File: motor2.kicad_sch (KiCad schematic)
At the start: 58 parts, among them IC5 DRV8300DPWR, IC6 DRV8300DPWR, J10 Conn_01x01, J11 Conn_01x01, J12 Conn_01x01, J7 Conn_01x01, J8 Conn_01x01, J9 Conn_01x01, Q13 Q_NMOS, Q14 Q_NMOS, Q15 Q_NMOS, Q16 Q_NMOS, Q17 Q_NMOS, Q18 Q_NMOS, Q19 Q_NMOS, Q20 Q_NMOS, Q21 Q_NMOS, Q22 Q_NMOS, Q23 Q_NMOS, Q24 Q_NMOS

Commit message: affected footprints
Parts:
- C21, C23, C24, C25, C26, C27, C28, C29: footprint (none) -> Capacitor_SMD:C_0402_1005Metric
- J10, J11, J12, J7, J8, J9: footprint (none) -> TestPoint:TestPoint_Pad_2.0x2.0mm; now left out of the parts list
- Q13, Q14, Q15, Q16, Q17, Q18, Q19, Q20, Q21, Q22, Q23, Q24: footprint (none) -> ESCs:TRANS_NTMFS5C628NLT1G
- R42, R43, R44, R45, R46, R47, R48, R49, R50, R51, R52, R53, R54, R55, R56, R57, R58, R59, R60, R61, R62, R63, R64, R65, R66, R67, R68, R69, R70, R71: footprint (none) -> Resistor_SMD:R_0402_1005Metric
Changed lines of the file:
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@@
 			)
 		)
-		(property "Footprint" ""
+		(property "Footprint" "Resistor_SMD:R_0402_1005Metric"
 			(at 181.61 42.418 90)
 			(effects
@@
 			)
 		)
-		(property "Footprint" ""
+		(property "Footprint" "ESCs:TRANS_NTMFS5C628NLT1G"
 			(at 129.54 130.81 0)
 			(effects
@@
 			)
 		)
-		(property "Footprint" ""
+		(property "Footprint" "ESCs:TRANS_NTMFS5C628NLT1G"
 			(at 129.54 115.57 0)
 			(effects
@@
 			)
 		)
-		(property "Footprint" ""
+		(property "Footprint" "Resistor_SMD:R_0402_1005Metric"
 			(at 66.548 71.12 90)
 			(effects
@@
 			)
 		)
-		(property "Footprint" ""
+		(property "Footprint" "Resistor_SMD:R_0402_1005Metric"
 			(at 112.268 81.28 90)
 			(effects
@@
 			)
 		)
-		(property "Footprint" ""
+		(property "Footprint" "Resistor_SMD:R_0402_1005Metric"
 			(at 157.48 135.128 90)
 			(effects
@@
 			)
 		)
-		(property "Footprint" ""
+		(property "Footprint" "Resistor_SMD:R_0402_1005Metric"
 			(at 199.39 119.888 90)
 			(effects
@@
 			)
 		)
-		(property "Footprint" ""
+		(property "Footprint" "ESCs:TRANS_NTMFS5C628NLT1G"
 			(at 214.63 115.57 0)
 			(effects
@@
 			)
 		)
-		(property "Footprint" ""
+		(property "Footprint" "Resistor_SMD:R_0402_1005Metric"
 			(at 57.658 158.75 90)
 			(effects
@@
 			)
 		)
-		(property "Footprint" ""
+		(property "Footprint" "Resistor_SMD:R_0402_1005Metric"
 			(at 38.1 162.052 90)
 			(effects
@@
 			)
 		)
-		(property "Footprint" ""
+		(property "Footprint" "ESCs:TRANS_NTMFS5C628NLT1G"
 			(at 214.63 130.81 0)
 			(effects
@@
 		(unit 1)
 		(exclude_from_sim no)
-		(in_bom yes)
+		(in_bom no)
 		(on_board yes)
 		(dnp no)
@@
 			)
 		)
-		(property "Footprint" ""
+		(property "Footprint" "TestPoint:TestPoint_Pad_2.0x2.0mm"
 			(at 176.53 125.73 0)
 			(effects
@@
 			)
 		)
-		(property "Footprint" ""
+		(property "Footprint" "Resistor_SMD:R_0402_1005Metric"
 			(at 34.798 158.75 90)
 			(effects
@@
 			)
 		)
-		(property "Footprint" ""
+		(property "Footprint" "Capacitor_SMD:C_0402_1005Metric"
 			(at 85.09 105.7148 0)
 			(effects
@@
 			)
 		)
-		(property "Footprint" ""
+		(property "Footprint" "Capacitor_SMD:C_0402_1005Metric"
 			(at 85.09 113.3348 0)
 			(effects
@@
 			)
 		)
-		(property "Footprint" ""
+		(property "Footprint" "ESCs:TRANS_NTMFS5C628NLT1G"
 			(at 238.76 38.1 0)
 			(effects
@@
 			)
 		)
-		(property "Footprint" ""
+		(property "Footprint" "Resistor_SMD:R_0402_1005Metric"
 			(at 115.57 74.422 90)
 			(effects
@@
 		(unit 1)
 		(exclude_from_sim no)
-		(in_bom yes)
+		(in_bom no)
 		(on_board yes)
 		(dnp no)
@@
 			)
 		)
-		(property "Footprint" ""
+		(property "Footprint" "TestPoint:TestPoint_Pad_2.0x2.0mm"
 			(at 200.66 48.26 0)
 			(effects
@@
 			)
 		)
-		(property "Footprint" ""
+		(property "Footprint" "Resistor_SMD:R_0402_1005Metric"
 			(at 60.96 162.052 90)
 			(effects
@@
 		(unit 1)
 		(exclude_from_sim no)
-		(in_bom yes)
+		(in_bom no)
 		(on_board yes)
 		(dnp no)
@@
 			)
 		)
-		(property "Footprint" ""
+		(property "Footprint" "TestPoint:TestPoint_Pad_2.0x2.0mm"
 			(at 133.35 125.73 0)
 			(effects
@@
 		(unit 1)
 		(exclude_from_sim no)
-		(in_bom yes)
+		(in_bom no)
 		(on_board yes)
 		(dnp no)
@@
 			)
 		)
-		(property "Footprint" ""
+		(property "Footprint" "TestPoint:TestPoint_Pad_2.0x2.0mm"
 			(at 218.44 125.73 0)
 			(effects
@@
 			)
 		)
-		(property "Footprint" ""
+		(property "Footprint" "Resistor_SMD:R_0402_1005Metric"
 			(at 157.48 119.888 90)
 			(effects
@@
 			)
 		)
-		(property "Footprint" ""
+		(property "Footprint" "ESCs:TRANS_NTMFS5C628NLT1G"
 			(at 153.67 38.1 0)
 			(effects
@@
 			)
 		)
-		(property "Footprint" ""
+		(property "Footprint" "Resistor_SMD:R_0402_1005Metric"
 			(at 57.658 168.91 90)
 			(effects
@@
 			)
 		)
-		(property "Footprint" ""
+		(property "Footprint" "Resistor_SMD:R_0402_1005Metric"
 			(at 138.43 42.418 90)
 			(effects
@@
 			)
 		)
-		(property "Footprint" ""
+		(property "Footprint" "Resistor_SMD:R_0402_1005Metric"
 			(at 80.518 168.91 90)
 			(effects
@@
 			)
 		)
-		(property "Footprint" ""
+		(property "Footprint" "Resistor_SMD:R_0402_1005Metric"
 			(at 114.3 135.128 90)
 			(effects
@@
 			)
 		)
-		(property "Footprint" ""
+		(property "Footprint" "Resistor_SMD:R_0402_1005Metric"
 			(at 89.408 81.28 90)
 			(effects
@@
 			)
 		)
-		(property "Footprint" ""
+		(property "Footprint" "ESCs:TRANS_NTMFS5C628NLT1G"
 			(at 153.67 53.34 0)
 			(effects
@@
 			)
 		)
-		(property "Footprint" ""
+		(property "Footprint" "Resistor_SMD:R_0402_1005Metric"
 			(at 112.268 71.12 90)
 			(effects
@@
 		(unit 1)
 		(exclude_from_sim no)
-		(in_bom yes)
+		(in_bom no)
 		(on_board yes)
 		(dnp no)
@@
 			)
 		)
-		(property "Footprint" ""
+		(property "Footprint" "TestPoint:TestPoint_Pad_2.0x2.0mm"
 			(at 157.48 48.26 0)
 			(effects
@@
 			)
 		)
-		(property "Footprint" ""
+		(property "Footprint" "ESCs:TRANS_NTMFS5C628NLT1G"
 			(at 238.76 53.34 0)
 			(effects
@@
 			)
 		)
-		(property "Footprint" ""
+		(property "Footprint" "Resistor_SMD:R_0402_1005Metric"
 			(at 223.52 42.418 90)
 			(effects
@@
 			)
 		)
-		(property "Footprint" ""
+		(property "Footprint" "ESCs:TRANS_NTMFS5C628NLT1G"
 			(at 196.85 38.1 0)
 			(effects
@@
 			)
 		)
-		(property "Footprint" ""
+		(property "Footprint" "Resistor_SMD:R_0402_1005Metric"
 			(at 34.798 168.91 90)
 			(effects
@@
 			)
 		)
-		(property "Footprint" ""
+		(property "Footprint" "Resistor_SMD:R_0402_1005Metric"
 			(at 138.43 57.658 90)
 			(effects
@@
 			)
 		)
-		(property "Footprint" ""
+		(property "Footprint" "Resistor_SMD:R_0402_1005Metric"
 			(at 89.408 71.12 90)
 			(effects
@@
 			)
 		)
-		(property "Footprint" ""
+		(property "Footprint" "Resistor_SMD:R_0402_1005Metric"
 			(at 66.548 81.28 90)
 			(effects
@@
 			)
 		)
-		(property "Footprint" ""
+		(property "Footprint" "Capacitor_SMD:C_0402_1005Metric"
 			(at 78.74 26.9748 0)
 			(effects
@@
 			)
 		)
-		(property "Footprint" ""
+		(property "Footprint" "Capacitor_SMD:C_0402_1005Metric"
 			(at 78.74 42.2148 0)
 			(effects
@@
 			)
 		)
-		(property "Footprint" ""
+		(property "Footprint" "Capacitor_SMD:C_0402_1005Metric"
 			(at 78.74 34.5948 0)
 			(effects
@@
 			)
 		)
-		(property "Footprint" ""
+		(property "Footprint" "ESCs:TRANS_NTMFS5C628NLT1G"
 			(at 172.72 130.81 0)
 			(effects
@@
 			)
 		)
-		(property "Footprint" ""
+		(property "Footprint" "ESCs:TRANS_NTMFS5C628NLT1G"
 			(at 196.85 53.34 0)
 			(effects
@@
 			)
 		)
-		(property "Footprint" ""
+		(property "Footprint" "Capacitor_SMD:C_0402_1005Metric"
 			(at 27.6352 52.07 0)
 			(effects
@@
 			)
 		)
-		(property "Footprint" ""
+		(property "Footprint" "Resistor_SMD:R_0402_1005Metric"
 			(at 80.518 158.75 90)
 			(effects
@@
 			)
 		)
-		(property "Footprint" ""
+		(property "Footprint" "Capacitor_SMD:C_0402_1005Metric"
 			(at 32.7152 130.81 0)
 			(effects
@@
 			)
 		)
-		(property "Footprint" ""
+		(property "Footprint" "ESCs:TRANS_NTMFS5C628NLT1G"
 			(at 172.72 115.57 0)
 			(effects
@@
 			)
 		)
-		(property "Footprint" ""
+		(property "Footprint" "Resistor_SMD:R_0402_1005Metric"
 			(at 83.82 162.052 90)
 			(effects
@@
 		(unit 1)
 		(exclude_from_sim no)
-		(in_bom yes)
+		(in_bom no)
 		(on_board yes)
 		(dnp no)
@@
 			)
 		)
-		(property "Footprint" ""
+		(property "Footprint" "TestPoint:TestPoint_Pad_2.0x2.0mm"
 			(at 242.57 48.26 0)
 			(effects
@@
 			)
 		)
-		(property "Footprint" ""
+		(property "Footprint" "Resistor_SMD:R_0402_1005Metric"
 			(at 114.3 119.888 90)
 			(effects
@@
 			)
 		)
-		(property "Footprint" ""
+		(property "Footprint" "Resistor_SMD:R_0402_1005Metric"
 			(at 92.71 74.422 90)
 			(effects
@@
 			)
 		)
-		(property "Footprint" ""
+		(property "Footprint" "Capacitor_SMD:C_0402_1005Metric"
 			(at 85.09 120.9548 0)
 			(effects
@@
 			)
 		)
-		(property "Footprint" ""
+		(property "Footprint" "Resistor_SMD:R_0402_1005Metric"
 			(at 69.85 74.422 90)
 			(effects
@@
 			)
 		)
-		(property "Footprint" ""
+		(property "Footprint" "Resistor_SMD:R_0402_1005Metric"
 			(at 181.61 57.658 90)
 			(effects
@@
 			)
 		)
-		(property "Footprint" ""
+		(property "Footprint" "Resistor_SMD:R_0402_1005Metric"
 			(at 199.39 135.128 90)
 			(effects
@@
 			)
 		)
-		(property "Footprint" ""
+		(property "Footprint" "Resistor_SMD:R_0402_1005Metric"
 			(at 223.52 57.658 90)
 			(effects

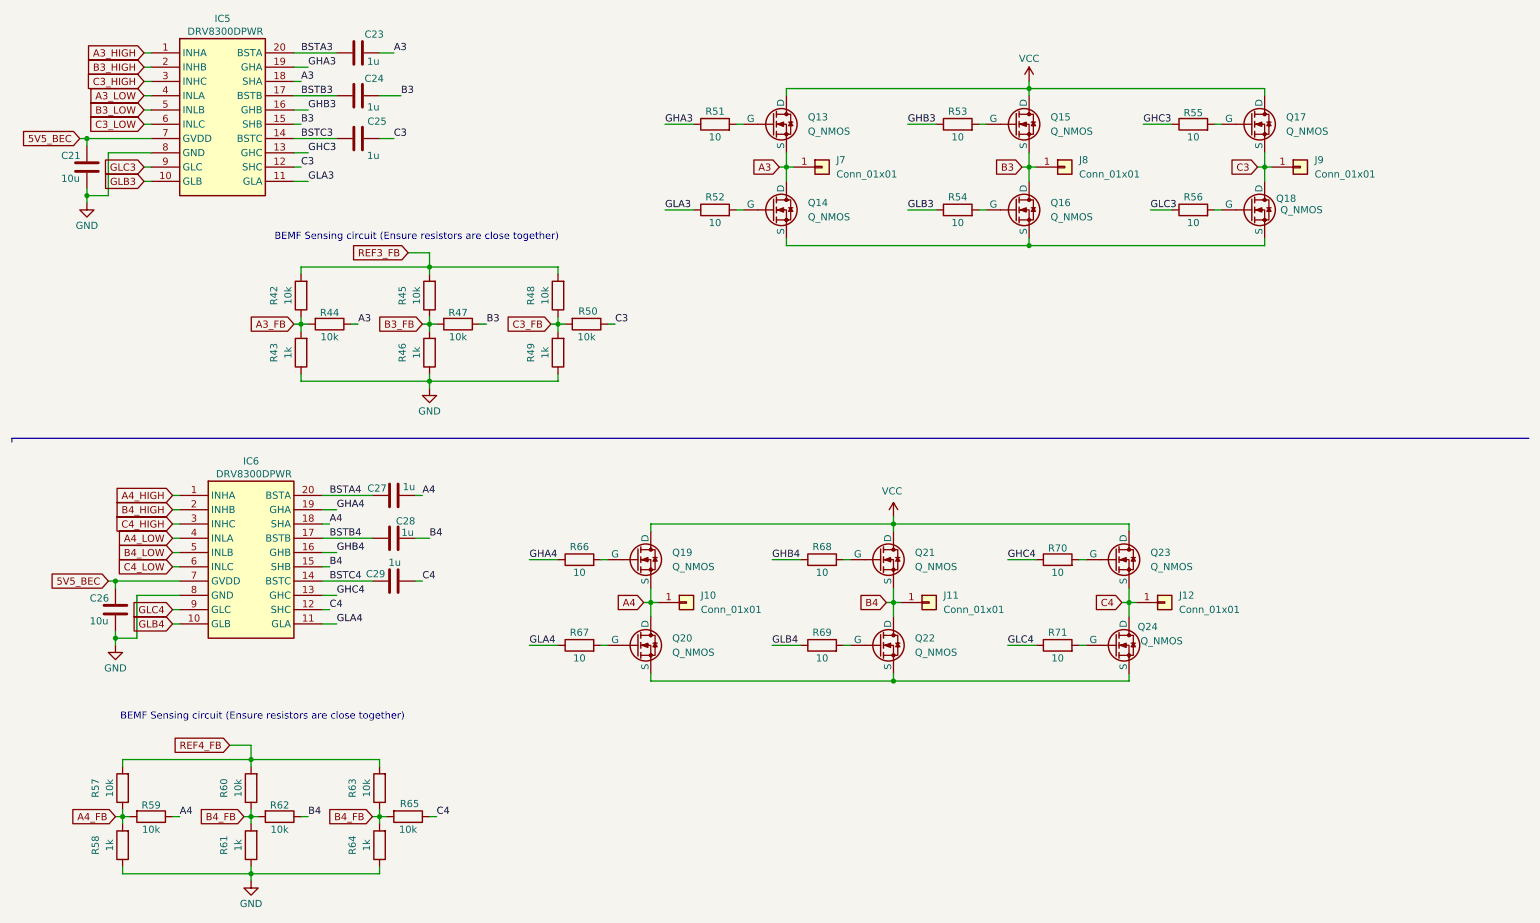
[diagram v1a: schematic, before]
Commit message: minor fixes
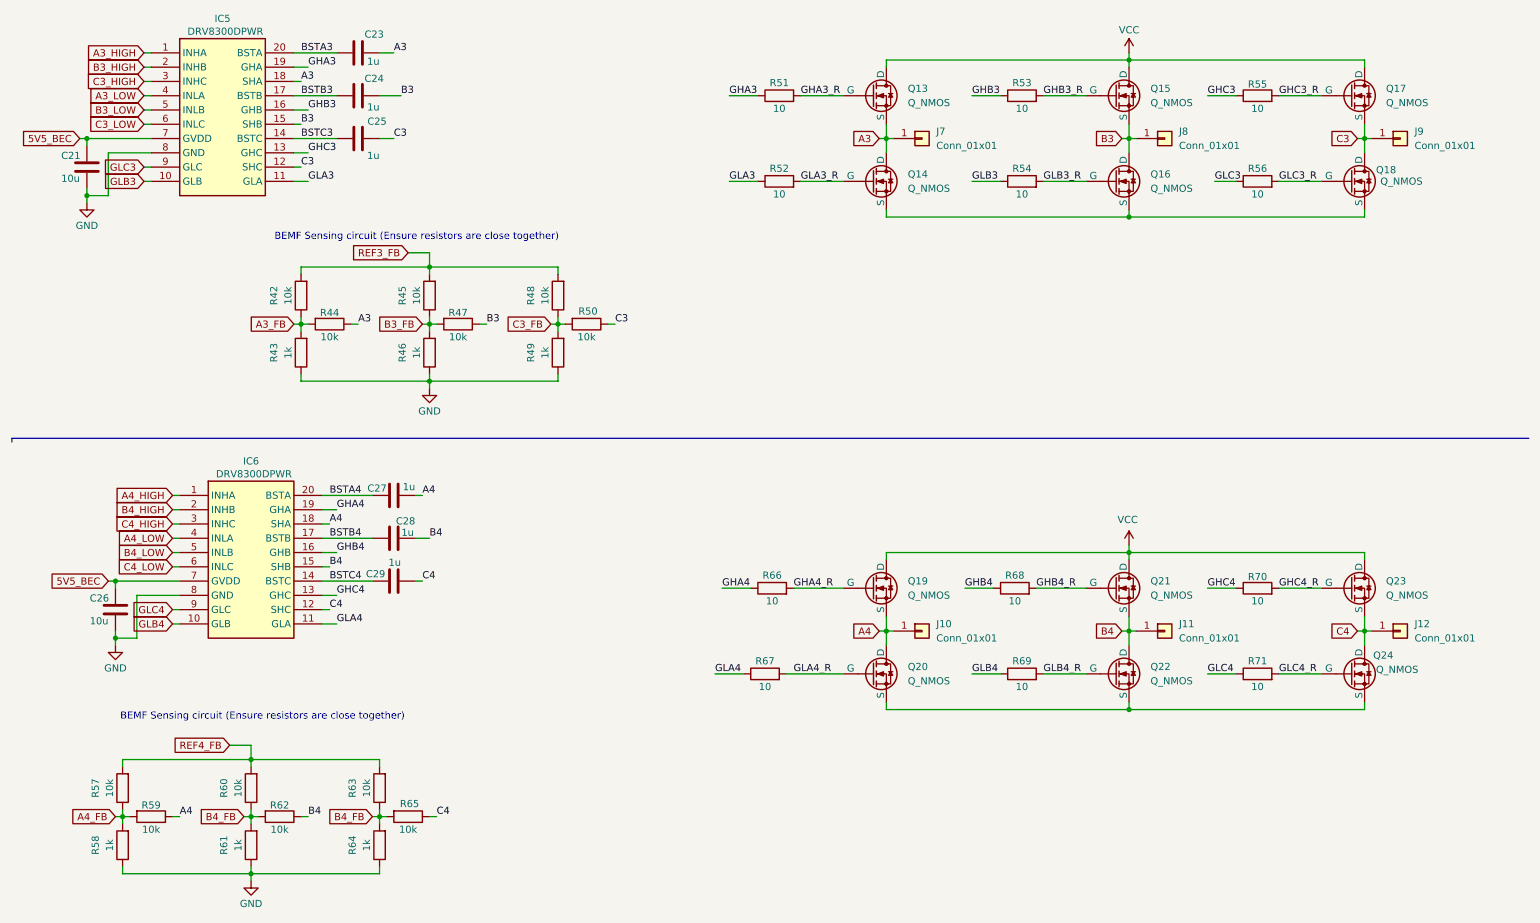
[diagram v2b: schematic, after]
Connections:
- net GHB3_R: now reaches Q15.G, R53.2
- net GLA4_R: now reaches Q20.G, R67.2
- net GHA4_R: now reaches Q19.G, R66.2
- net GLB4_R: now reaches Q22.G, R69.2
- net GHC4_R: now reaches Q23.G, R70.2
- net GLC4_R: now reaches Q24.G, R71.2
- net GHC3_R: now reaches Q17.G, R55.2
- net GHB4_R: now reaches Q21.G, R68.2
- net GHA3_R: now reaches Q13.G, R51.2
- net GLA3_R: now reaches Q14.G, R52.2
- net GLC3_R: now reaches Q18.G, R56.2
- net GLB3_R: now reaches Q16.G, R54.2
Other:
- moved on the sheet: J10, J11, J12, J7, J8, J9, Q13, Q14, Q15, Q16, Q17, Q18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
